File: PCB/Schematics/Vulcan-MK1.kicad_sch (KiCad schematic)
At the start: 0 parts

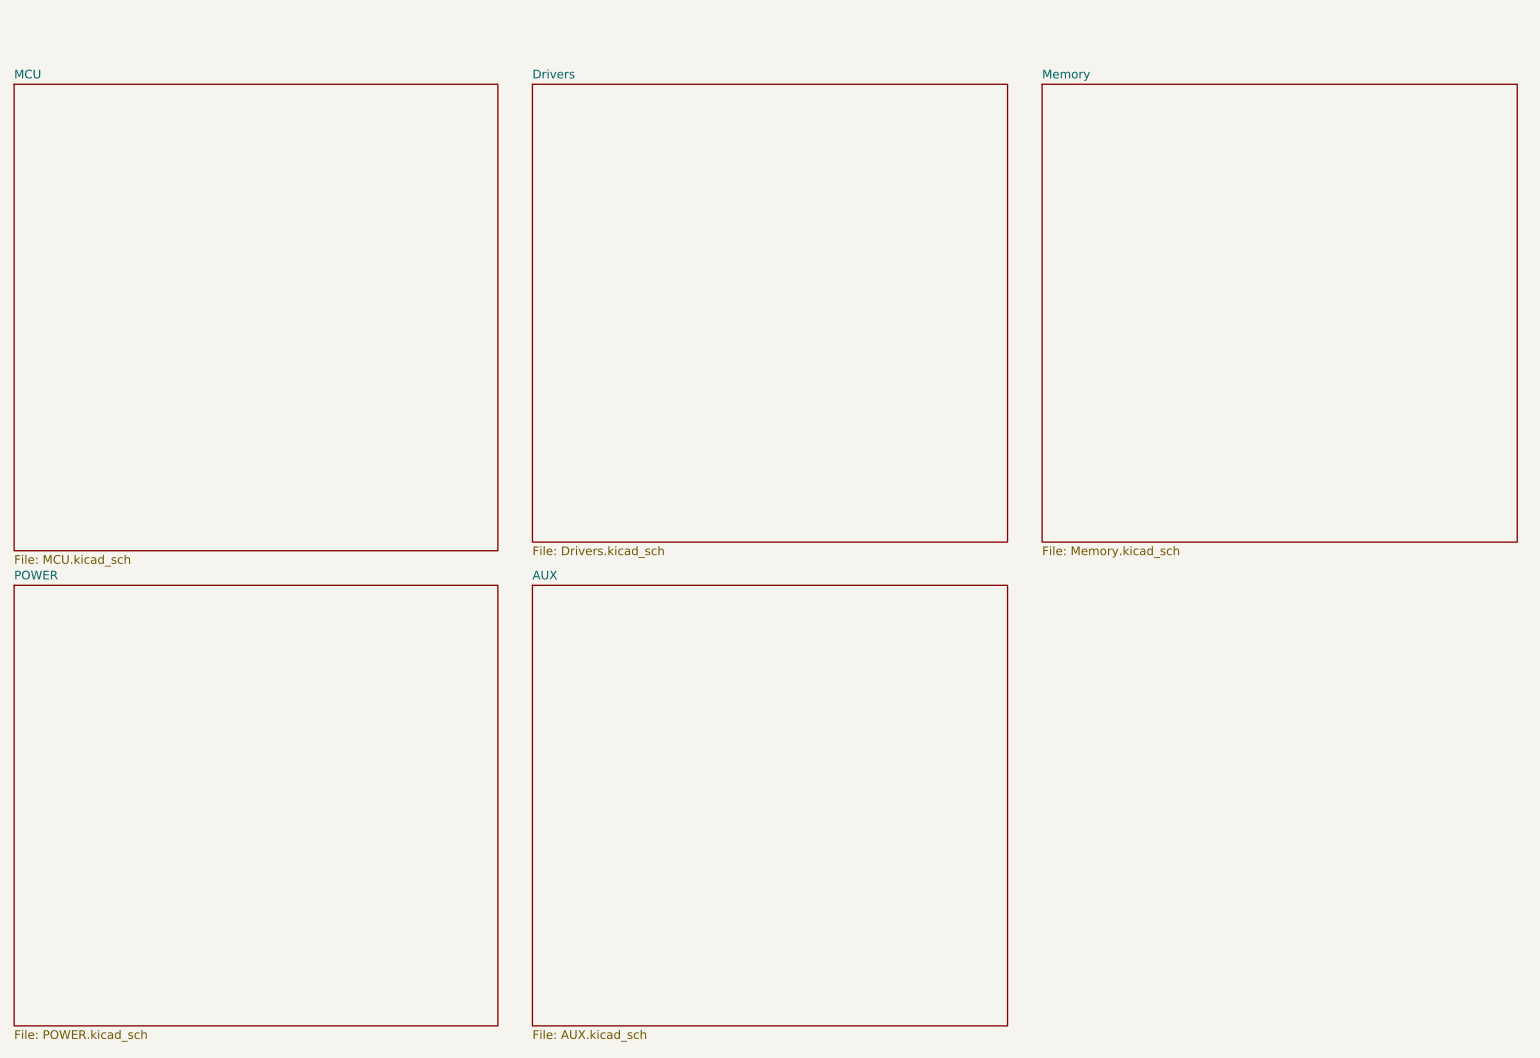
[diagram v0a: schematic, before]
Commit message: Add changes
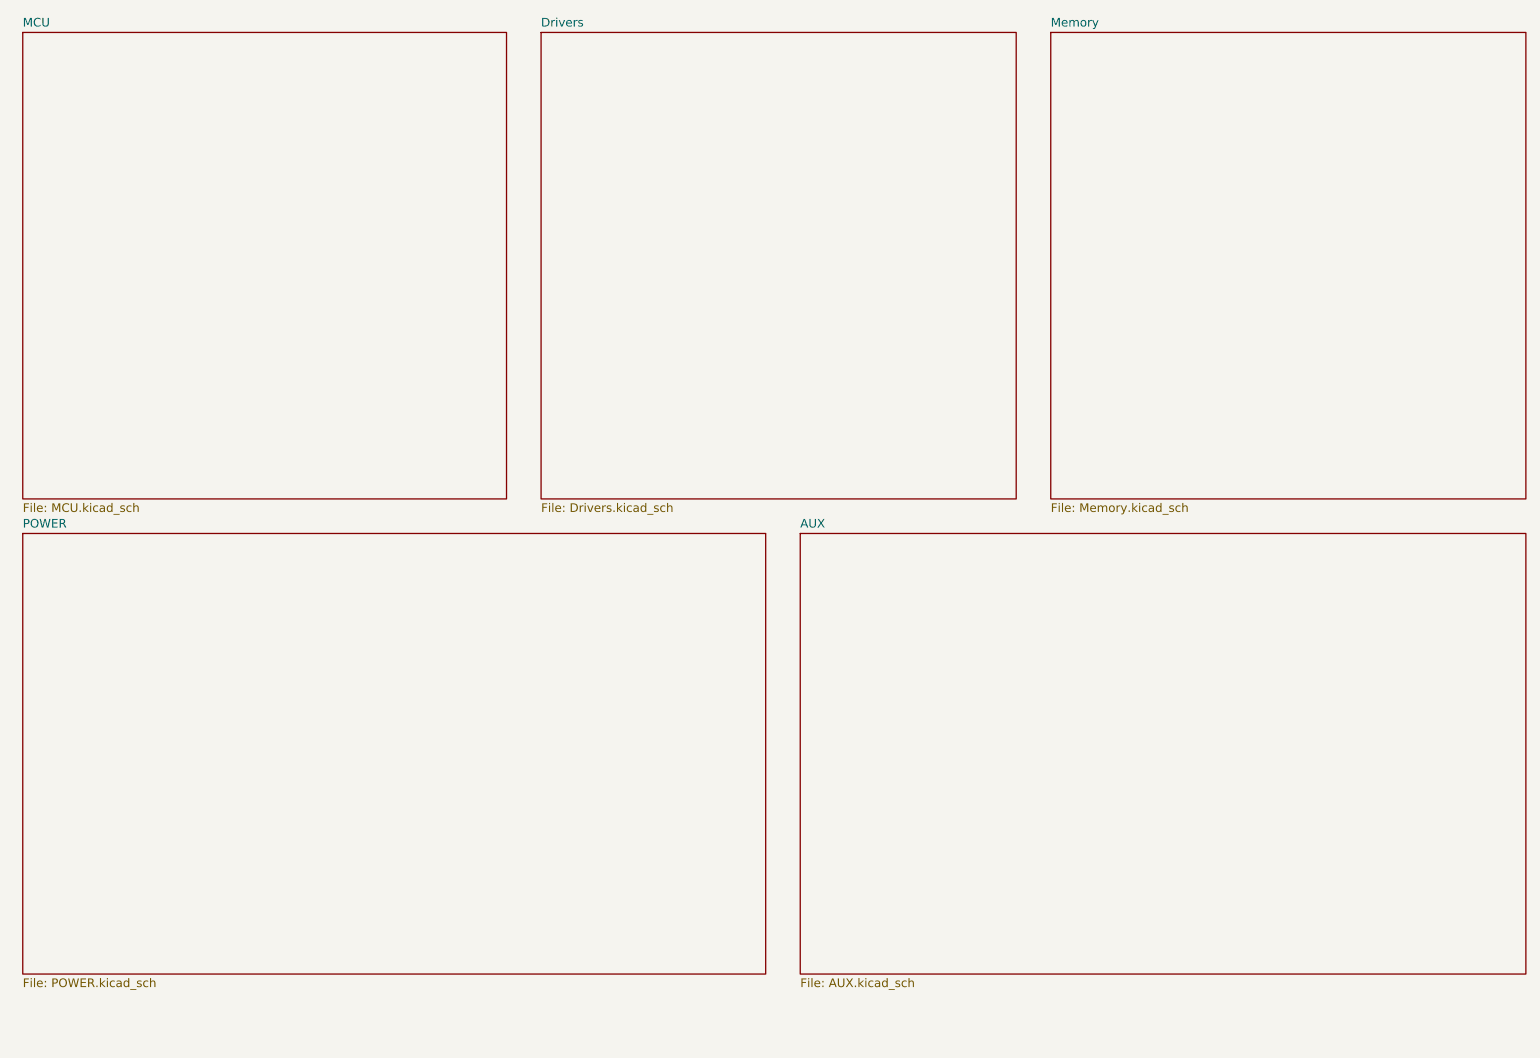
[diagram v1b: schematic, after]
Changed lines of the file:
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@@
 	(paper "A4")
 	(sheet
-		(at 110.49 31.75)
-		(size 69.85 67.31)
+		(at 111.76 24.13)
+		(size 69.85 68.58)
 		(exclude_from_sim no)
 		(in_bom yes)
@@
 		)
 		(property "Sheetname" "Drivers"
-			(at 110.49 31.0384 0)
+			(at 111.76 23.4184 0)
 			(effects
 				(font
@@
 		)
 		(property "Sheetfile" "Drivers.kicad_sch"
-			(at 110.49 99.6446 0)
+			(at 111.76 93.2946 0)
 			(effects
 				(font
@@
 	)
 	(sheet
-		(at 185.42 31.75)
-		(size 69.85 67.31)
+		(at 186.69 24.13)
+		(size 69.85 68.58)
 		(exclude_from_sim no)
 		(in_bom yes)
@@
 		)
 		(property "Sheetname" "Memory"
-			(at 185.42 31.0384 0)
+			(at 186.69 23.4184 0)
 			(effects
 				(font
@@
 		)
 		(property "Sheetfile" "Memory.kicad_sch"
-			(at 185.42 99.6446 0)
+			(at 186.69 93.2946 0)
 			(effects
 				(font
@@
 	)
 	(sheet
-		(at 34.29 31.75)
+		(at 35.56 24.13)
 		(size 71.12 68.58)
 		(exclude_from_sim no)
@@
 		)
 		(property "Sheetname" "MCU"
-			(at 34.29 31.0384 0)
+			(at 35.56 23.4184 0)
 			(effects
 				(font
@@
 		)
 		(property "Sheetfile" "MCU.kicad_sch"
-			(at 34.29 100.9146 0)
+			(at 35.56 93.2946 0)
 			(effects
 				(font
@@
 	)
 	(sheet
-		(at 34.29 105.41)
-		(size 71.12 64.77)
+		(at 35.56 97.79)
+		(size 109.22 64.77)
 		(exclude_from_sim no)
 		(in_bom yes)
@@
 		)
 		(property "Sheetname" "POWER"
-			(at 34.29 104.6984 0)
+			(at 35.56 97.0784 0)
 			(effects
 				(font
@@
 		)
 		(property "Sheetfile" "POWER.kicad_sch"
-			(at 34.29 170.7646 0)
+			(at 35.56 163.1446 0)
 			(effects
 				(font
@@
 	)
 	(sheet
-		(at 110.49 105.41)
-		(size 69.85 64.77)
+		(at 149.86 97.79)
+		(size 106.68 64.77)
 		(exclude_from_sim no)
 		(in_bom yes)
@@
 		)
 		(property "Sheetname" "AUX"
-			(at 110.49 104.6984 0)
+			(at 149.86 97.0784 0)
 			(effects
 				(font
@@
 		)
 		(property "Sheetfile" "AUX.kicad_sch"
-			(at 110.49 170.7646 0)
+			(at 149.86 163.1446 0)
 			(effects
 				(font
